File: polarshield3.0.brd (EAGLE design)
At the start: 100 x 80 mm, 2 parts

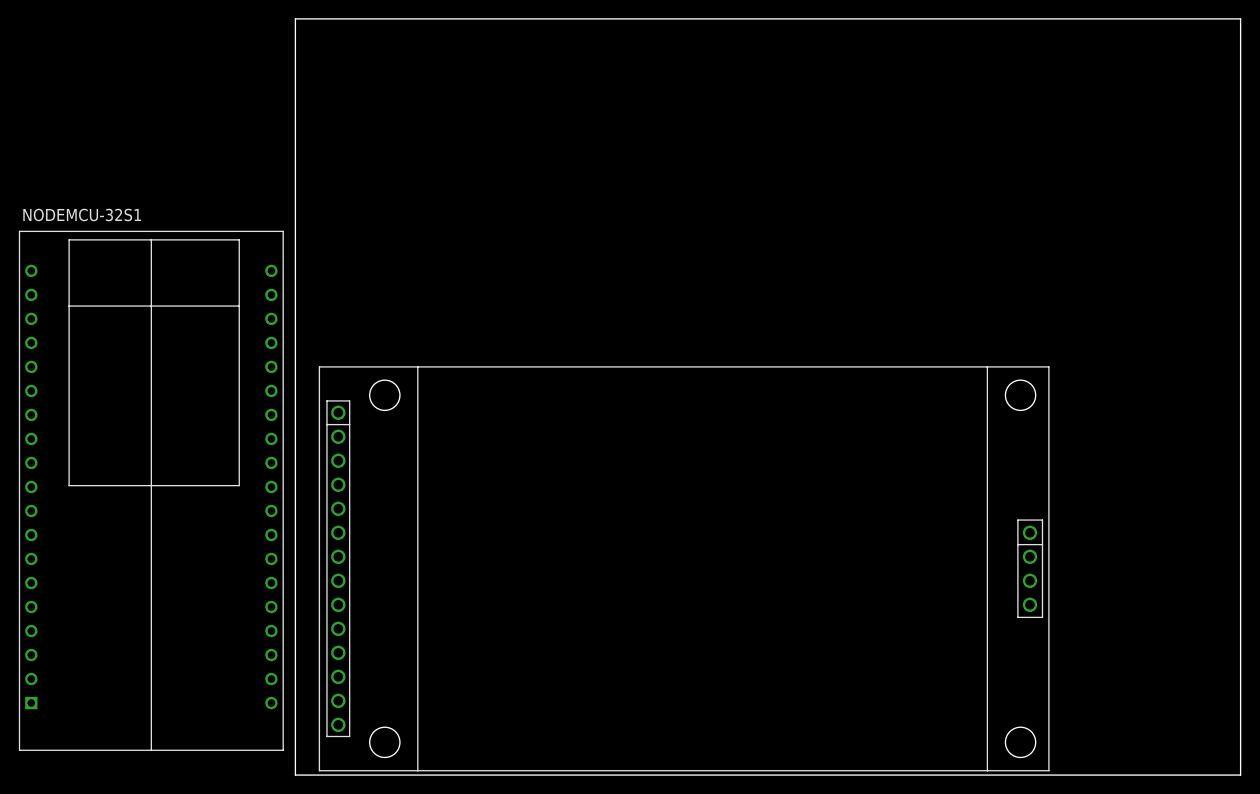
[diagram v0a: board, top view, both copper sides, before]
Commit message: first version looks ok visually
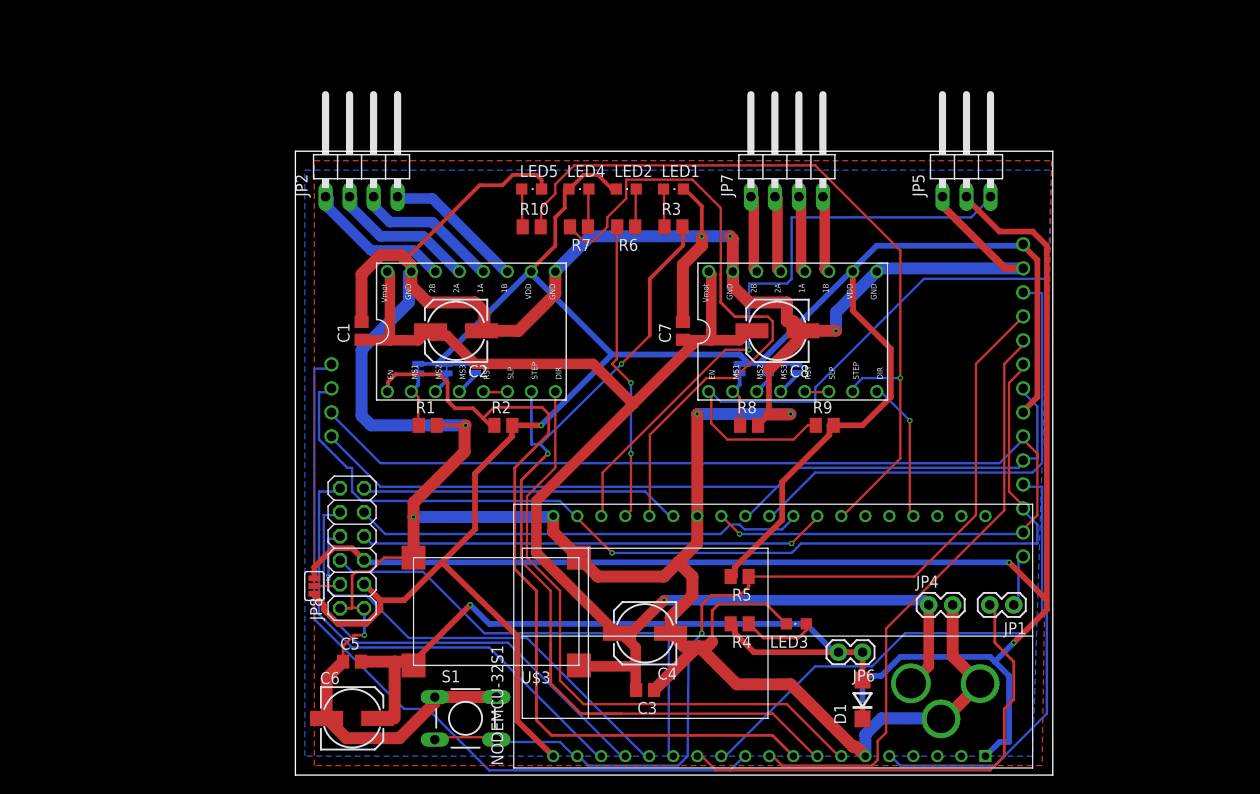
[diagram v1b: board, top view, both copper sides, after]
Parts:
- added C1, C7: (no value), resistor:C0805
- added C2, C8: (no value), resistor:153CLV-0605
- added C3, C5: 100nF, resistor:C0805
- added C4, C6: 220uF, resistor:153CLV-0605
- added D1: (no value), diode:DO214BA
- added JP1, JP4, JP6: (no value), SparkFun-Connectors:1X02
- added JP2, JP7: (no value), pinhead:1X04/90
- added JP3: POWER_JACKPTH_LOCK, SparkFun-Connectors:POWER_JACK_PTH_LOCK
- added JP5: (no value), pinhead:1X03/90
- added JP8: (no value), pinhead:2X06
- added LED1, LED2, LED3, LED4, LED5: (no value), polargraph3:CHIPLED_0805
- added R1, R10, R2, R3, R8, R9: (no value), resistor:M0805
- added R4, R5, R6, R7: 1k, resistor:M0805
- added S1: DTS-6, switch-tact:DTS-6
- added SJ1, SJ4: SOLDERJUMPERNO, polargraph3:SJ_2S-NO
- added SJ2, SJ3, SJ5, SJ6: SOLDERJUMPERTRACE, polargraph3:SJ_2S-TRACE
- added SJ7: (no value), SparkFun-Retired:SJ_3_PASTE1&2
- added U$1, U$4: A4988BREAKOUT, sandy:A4988BREAKOUT
- added U$3: MINI-360-MP2307, polargraph3:MINI-360-MP2307
- U$2: device sandy:2.4_TFT_SPI_TOUCH_SD -> polargraph3:2.4_TFT_SPI_TOUCH_SD
- moved NODEMCU-32S1 101.1 mm to (73.0, 2.00), turned to 90 degrees
- moved U$2 78.5 mm to (79.0, 61.0), flipped to the bottom
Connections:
- new net +12V: C1.1, C2.+, C3.2, C4.+, C7.1, C8.+, JP3.PWR, JP4.1, U$1.VMOT, U$3.+V_IN, U$4.VMOT
- new net ENC1_A: JP8.12, NODEMCU-32S1.SVP
- new net ENC1_B: JP8.10, NODEMCU-32S1.SVN
- new net ENC2_A: JP8.8, NODEMCU-32S1.P34
- new net ENC2_B: JP8.6, NODEMCU-32S1.P35
- new net GP_1: JP8.11, NODEMCU-32S1.P21
- new net GP_2: JP8.9, NODEMCU-32S1.P17
- new net GP_3: JP8.7, NODEMCU-32S1.P16
- new net M1_DIR: NODEMCU-32S1.P12, U$1.DIR
- new net M1_EN: NODEMCU-32S1.P27, R2.1, U$1.EN
- new net M1_STEP: NODEMCU-32S1.P14, R3.2, U$1.STEP
- new net M2_DIR: NODEMCU-32S1.P15, U$4.DIR
- new net M2_EN: NODEMCU-32S1.P13, R9.1, U$4.EN
- new net M2_STEP: NODEMCU-32S1.P4, R10.2, U$4.STEP
- new net N$1: JP1.2, NODEMCU-32S1.P32
- new net N$10: JP2.1, U$1.2B
- new net N$11: JP2.2, U$1.2A
- new net N$12: JP2.3, U$1.1A
- new net N$13: JP2.4, U$1.1B
- new net N$14: LED2.C, R6.1
- new net N$15: LED4.C, R7.1
- new net N$16: SJ5.2, U$4.MS2
- new net N$17: R8.1, SJ6.2, U$4.MS1
- new net N$18: U$4.RST, U$4.SLP
- new net N$19: LED5.A, R10.1
- new net N$2: U$1.RST, U$1.SLP
- new net N$20: JP7.1, U$4.2B
- new net N$21: JP7.2, U$4.2A
- new net N$22: JP7.3, U$4.1A
- new net N$23: JP7.4, U$4.1B
- new net N$28: JP8.4, SJ7.2
- new net N$3: SJ1.2, U$1.MS3
- new net N$4: SJ2.2, U$1.MS2
- new net N$5: R1.1, SJ3.2, U$1.MS1
- new net N$6: LED1.A, R3.1
- new net N$7: C5.2, C6.+, D1.A, JP6.1, JP6.2, R4.2, U$3.+V_OUT
- new net N$8: LED3.A, R4.1
- new net N$9: SJ4.2, U$4.MS3
- new net RESET: NODEMCU-32S1.EN, R5.1, S1.3, S1.4, U$2.RESET
- new net RX: NODEMCU-32S1.RX, R7.2
- new net SD_CS: NODEMCU-32S1.P25, U$2.SD_CS
- new net SERVO1: JP5.3, NODEMCU-32S1.P22
- new net SPI_CLK: NODEMCU-32S1.P18, U$2.SCK, U$2.SD_SCK, U$2.T_CLK
- new net SPI_MISO: NODEMCU-32S1.P19, U$2.SDO-MISO, U$2.SD_MISO, U$2.T_DO
- new net SPI_MOSI: NODEMCU-32S1.P23, U$2.SDI-MOSI, U$2.SD_MOSI, U$2.T_DIN
- new net TFT_CS: NODEMCU-32S1.P5, U$2.CS
- new net TFT_DC: NODEMCU-32S1.P26, U$2.D/C
- new net TX: NODEMCU-32S1.TX, R6.2
- new net T_CS: NODEMCU-32S1.P33, U$2.T_CS
- new net T_IRQ: JP1.1, U$2.T_IRQ
- net +3V3: now also JP8.3, LED2.A, LED4.A, R2.2, R5.2, R9.2, SJ1.1, SJ2.1, SJ3.1, SJ4.1, SJ5.1, SJ6.1, SJ7.3, U$1.VDD, U$2.LED, U$4.VDD
- net +5V: now also D1.C, JP5.2, JP8.5, SJ7.1
- net GND: now also C1.2, C2.-, C3.1, C4.-, C5.1, C6.-, C7.2, C8.-, JP3.GND, JP3.GNDBREAK, JP4.2, JP5.1, JP8.1, JP8.2, LED1.C, LED3.C, LED5.C, R1.2, R8.2, S1.1, S1.2, U$1.GND, U$1.GND@0, U$3.GND_IN, U$3.GND_OUT, U$4.GND, U$4.GND@0
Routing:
- net GND: track 0.00 -> 398.7 mm, vias 0 -> 8
- net +3V3: track 0.00 -> 243.5 mm, vias 0 -> 1
- net +5V: track 0.00 -> 170.7 mm, vias 0 -> 3
- net +12V: track 0.00 -> 154.1 mm, vias 0 -> 1
- net M2_EN: track 0.00 -> 123.8 mm
- net SPI_MISO: track 0.00 -> 121.1 mm, vias 0 -> 1
- net SPI_MOSI: track 0.00 -> 110.3 mm, vias 0 -> 1
- net RESET: track 0.00 -> 101.7 mm, vias 0 -> 1
- net M1_STEP: track 0.00 -> 95.7 mm, vias 0 -> 2
- net SPI_CLK: track 0.00 -> 91.2 mm
- net M1_EN: track 0.00 -> 87.3 mm
- net M2_STEP: track 0.00 -> 82.8 mm, vias 0 -> 1
- net N$7: track 0.00 -> 82.0 mm, vias 0 -> 1
- net SD_CS: track 0.00 -> 81.4 mm
- net RX: track 0.00 -> 66.6 mm
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- added copper zone on layer 1, net GND
- added copper zone on layer 16, net GND
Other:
- board size 100 x 80 mm -> 80.1 x 66 mm
